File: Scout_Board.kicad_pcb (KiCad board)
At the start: 2 copper layers, 87.4 x 67 mm, 3 parts, among them J10 BBAI_P8, J2 Conn_02x07_Odd_Even, J9 BBAI_P9

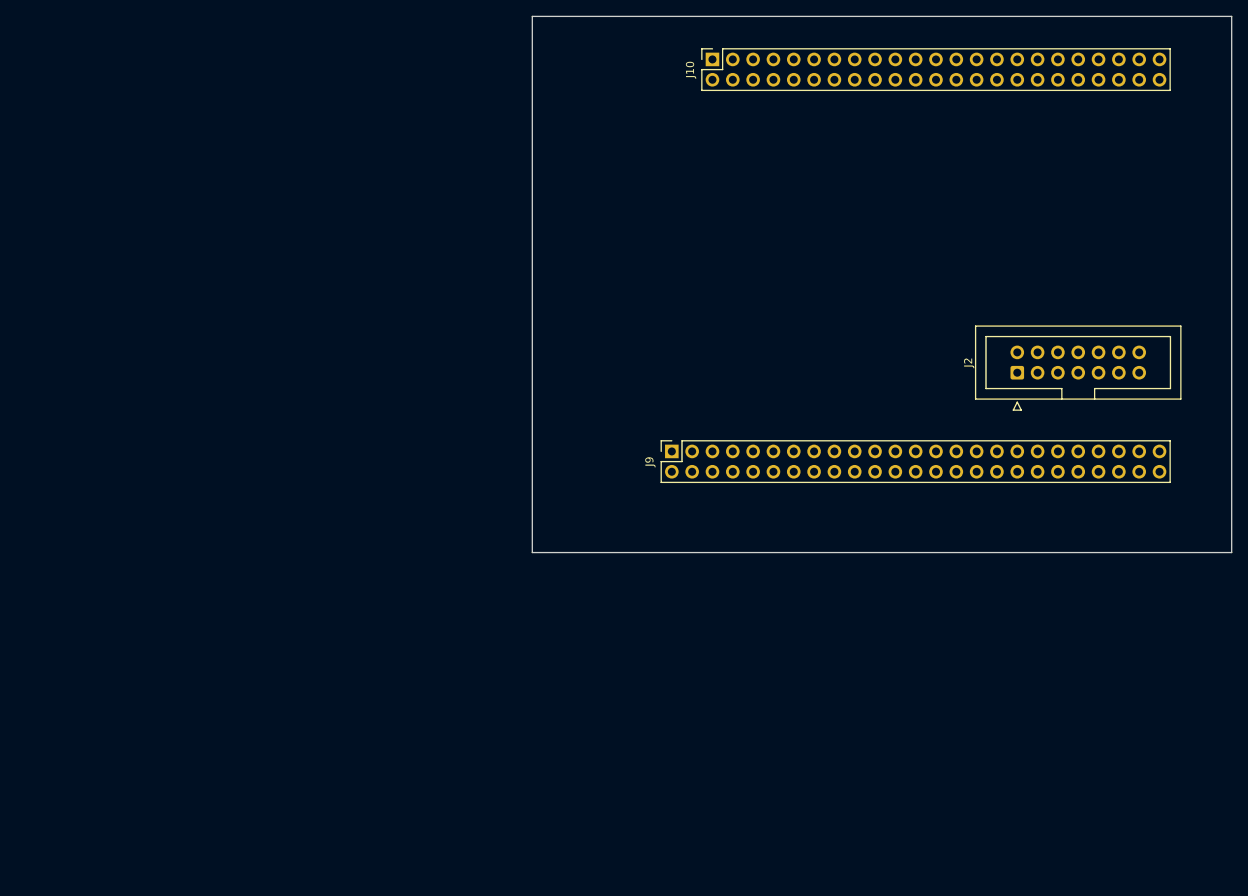
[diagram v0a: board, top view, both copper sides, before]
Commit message: New board test
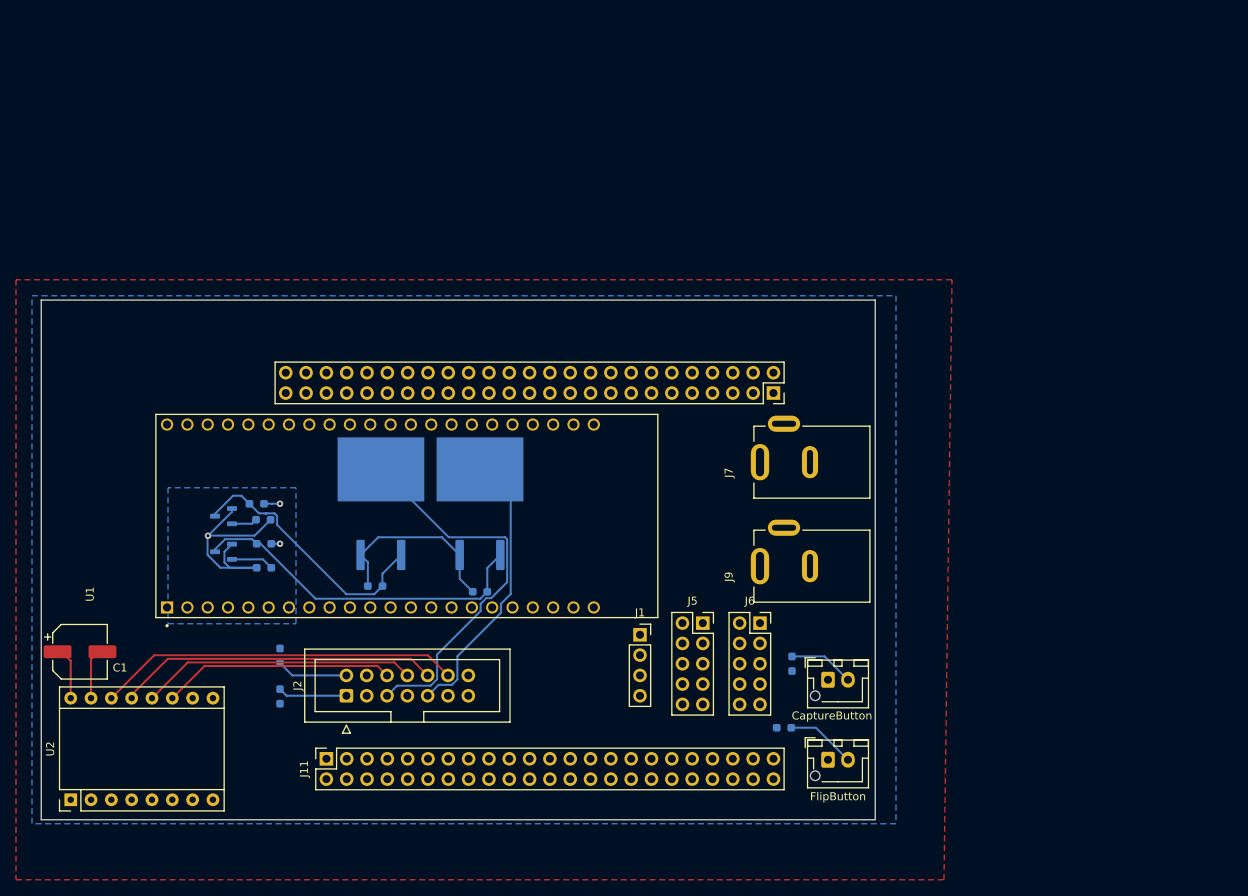
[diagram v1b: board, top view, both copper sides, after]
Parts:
- added C1: 100uF/16V, Capacitor_SMD:CP_Elec_6.3x5.9, F.Cu at (147.0, 169.5)
- added Conn2: CaptureButton, Connector_JST:JST_XH_B2B-XH-AM_1x02_P2.50mm_Vertical, F.Cu at (240.5, 173.0)
- added Conn4: FlipButton, Connector_JST:JST_XH_B2B-XH-AM_1x02_P2.50mm_Vertical, F.Cu at (240.5, 183.0)
- added J1: Conn_01x04_Pin, Connector_PinSocket_2.54mm:PinSocket_1x04_P2.54mm_Vertical, F.Cu at (217.0, 167.4)
- added J11: BBAI_P8, Connector_PinSocket_2.54mm:PinSocket_2x23_P2.54mm_Vertical, F.Cu at (177.8, 182.9)
- added J5: 5V, Connector_PinSocket_2.54mm:PinSocket_2x05_P2.54mm_Vertical, F.Cu at (224.8, 165.9)
- added J6: GND, Connector_PinSocket_2.54mm:PinSocket_2x05_P2.54mm_Vertical, F.Cu at (232.0, 165.9)
- added J7: IN, RAPC722X:SWITCHCRAFT_RAPC722X, F.Cu at (238.2, 145.8)
- added MOSFET1: IRFZ44NSTRLPBF, IRFZ44NSTRLPBF:DPAK254P1524X483-3N, B.Cu at (184.6, 151.0)
- added MOSFET2: IRFZ44NSTRLPBF, IRFZ44NSTRLPBF:DPAK254P1524X483-3N, B.Cu at (197.0, 151.0)
- added Q1: BSS138, BSS138:SOT95P240X111-3N, B.Cu at (164.9, 152.6)
- added Q2: BSS138, BSS138:SOT95P240X111-3N, B.Cu at (164.9, 157.0)
- added R1: 10k, Resistor_SMD:R_0603_1608Metric_Pad0.98x0.95mm_HandSolder, B.Cu at (235.0, 179.0)
- added R10: 1M, Resistor_SMD:R_0603_1608Metric_Pad0.98x0.95mm_HandSolder, B.Cu at (183.9, 161.3)
- added R11: 10k, Resistor_SMD:R_0603_1608Metric_Pad0.98x0.95mm_HandSolder, B.Cu at (169.1, 151.0)
- added R12: 10k, Resistor_SMD:R_0603_1608Metric_Pad0.98x0.95mm_HandSolder, B.Cu at (170.0, 159.0)
- added R13: 1M, Resistor_SMD:R_0603_1608Metric_Pad0.98x0.95mm_HandSolder, B.Cu at (197.0, 162.0)
- added R14: 10k, Resistor_SMD:R_0603_1608Metric_Pad0.98x0.95mm_HandSolder, B.Cu at (170.0, 156.0)
- added R2: 10k, Resistor_SMD:R_0603_1608Metric_Pad0.98x0.95mm_HandSolder, B.Cu at (236.0, 171.0)
- added R7: 10k, Resistor_SMD:R_0603_1608Metric_Pad0.98x0.95mm_HandSolder, B.Cu at (172.0, 175.1)
- added R8: 10k, Resistor_SMD:R_0603_1608Metric_Pad0.98x0.95mm_HandSolder, B.Cu at (172.0, 170.0)
- added R9: 10k, Resistor_SMD:R_0603_1608Metric_Pad0.98x0.95mm_HandSolder, B.Cu at (169.9, 153.0)
- added U1: ESP32-S3-DEVKITC-1U-N8R2, ESP32-S3-DEVKITC-1-N8R2:XCVR_ESP32-S3-DEVKITC-1-N8R2, F.Cu at (187.9, 152.5)
- added U2: ~, Module:Pololu_Breakout-16_15.2x20.3mm, F.Cu at (145.8, 188.0)
- J10: value BBAI_P8 -> BBAI_P9; footprint Connector_PinSocket_2.54mm:PinSocket_2x23_P2.54mm_Vertical -> Connector_PinSocket_2.54mm:PinSocket_2x25_P2.54mm_Vertical
- J9: value BBAI_P9 -> IN; footprint Connector_PinSocket_2.54mm:PinSocket_2x25_P2.54mm_Vertical -> RAPC722X:SWITCHCRAFT_RAPC722X
- moved J2 93.1 mm to (180.3, 175.0)
- moved J10 42.4 mm to (233.7, 137.2), turned to -90 degrees
- moved J9 22.4 mm to (238.2, 158.8)
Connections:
- net BLb renamed +12V
- J2 pad 3: Sw1b -> 5V
- J2 pad 4: Sw1b -> 5V
- J9 pad 1: unconnected-(J9-GND-Pad1) -> 5V
- J9 pad 2: unconnected-(J9-GND-Pad2) -> GND
- J9 pad 3: unconnected-(J9-3.3V-Pad3) -> GND
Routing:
- net TLa: track 0.00 -> 48.0 mm
- net 2B: track 0.00 -> 45.3 mm
- net BottomLightsHV: track 0.00 -> 43.6 mm
- net 2A: track 0.00 -> 40.1 mm
- net BLa: track 0.00 -> 35.2 mm
- net 1A: track 0.00 -> 34.4 mm
- net TopLightsHV: track 0.00 -> 33.2 mm
- net GND: track 0.00 -> 30.7 mm
- net +3.3V: track 0.00 -> 29.5 mm, vias 0 -> 1
- net 1B: track 0.00 -> 29.0 mm
- net Sw2: track 0.00 -> 8.94 mm
- net FlipButton: track 0.00 -> 8.74 mm
- net Sw1: track 0.00 -> 8.64 mm
- net CaptureButton: track 0.00 -> 8.21 mm
- net +12V: track 0.00 -> 6.98 mm
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- added copper zone on F.Cu, net +12V
- added copper zone on B.Cu, net +3.3V
- added copper zone on In1.Cu, net +3.3V
- added copper zone on In2.Cu, net 5V
- added copper zone on B.Cu, net GND
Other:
- board size 87.4 x 67 mm -> 104.2 x 65 mm
- copper layers 2 -> 4

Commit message: Layout changes
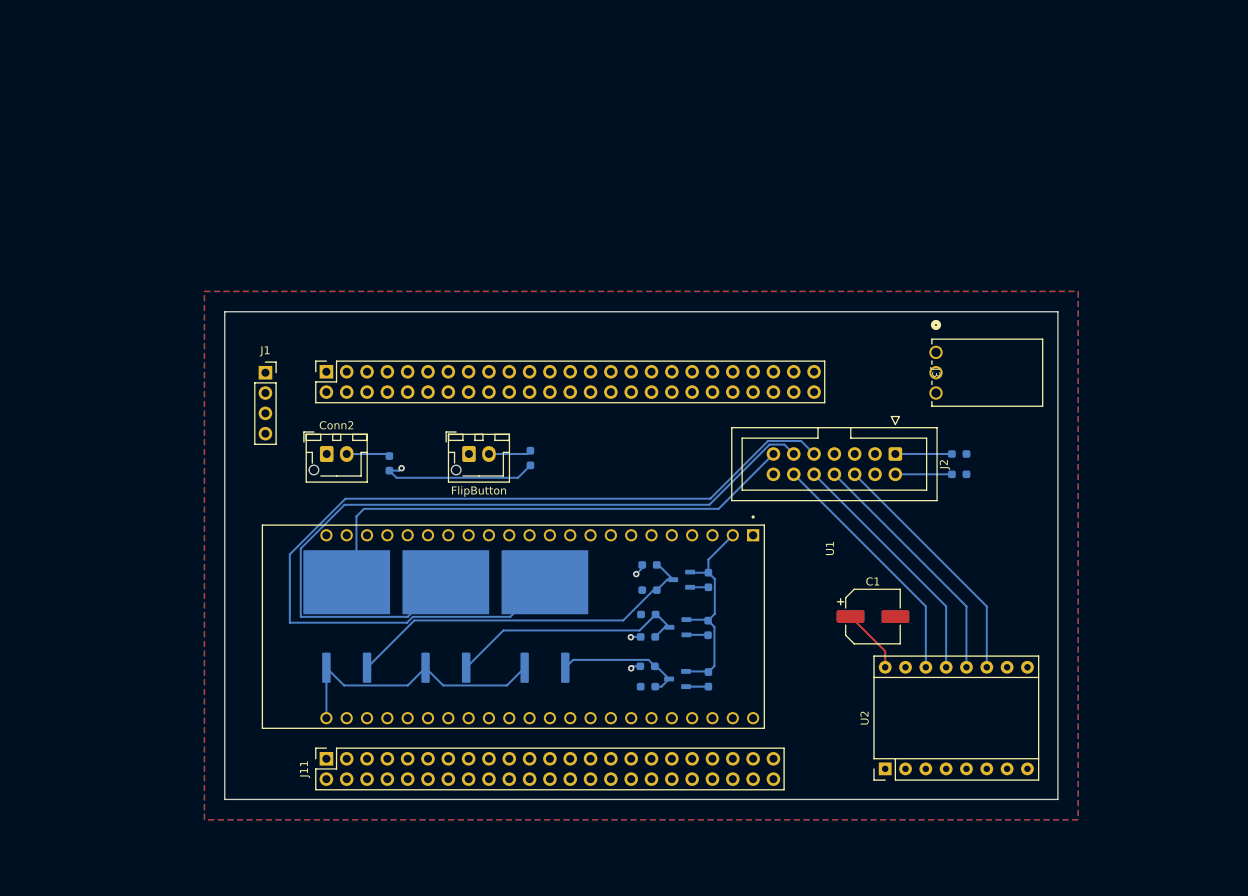
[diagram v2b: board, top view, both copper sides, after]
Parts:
- removed J5: 5V, Connector_PinSocket_2.54mm:PinSocket_2x05_P2.54mm_Vertical
- removed J6: GND, Connector_PinSocket_2.54mm:PinSocket_2x05_P2.54mm_Vertical
- removed J7, J9: IN, RAPC722X:SWITCHCRAFT_RAPC722X
- added J3: 705530002, 705530002:CONN3_53-0002_MOL, F.Cu at (254.0, 132.1)
- added MOSFET3: IRFZ44NSTRLPBF, IRFZ44NSTRLPBF:DPAK254P1524X483-3N, B.Cu at (180.3, 165.1)
- added Q3: BSS138, BSS138:SOT95P240X111-3N, B.Cu at (222.2, 160.5)
- added R29: 10k, Resistor_SMD:R_0603_1608Metric_Pad0.98x0.95mm_HandSolder, B.Cu at (225.6, 160.5)
- added R30: 1M, Resistor_SMD:R_0603_1608Metric_Pad0.98x0.95mm_HandSolder, B.Cu at (218.2, 158.6)
- added R31: 10k, Resistor_SMD:R_0603_1608Metric_Pad0.98x0.95mm_HandSolder, B.Cu at (218.2, 161.8)
- moved U2 101.9 mm to (247.7, 184.1)
- moved C1 99.2 mm to (246.1, 165.1)
- moved R7 90.1 mm to (256.9, 144.8), turned to 0 degrees
- moved R8 87.9 mm to (256.9, 147.3), turned to 0 degrees
- moved J2 75.0 mm to (248.9, 144.8), turned to -90 degrees
- moved Conn2 68.7 mm to (177.8, 144.8)
- moved Q1 60.3 mm to (221.7, 172.9)
- moved R9 59.1 mm to (225.6, 172.9), turned to -90 degrees
- moved Conn4 58.9 mm to (195.6, 144.8)
- moved Q2 57.6 mm to (221.7, 166.4)
- moved J1 57.1 mm to (170.2, 134.6)
- moved R2 56.2 mm to (185.7, 145.9)
- moved R12 56.0 mm to (225.5, 166.5), turned to -90 degrees
- moved J10 55.9 mm to (177.8, 134.5), turned to 90 degrees
- moved R11 54.0 mm to (218.0, 173.9), turned to 0 degrees
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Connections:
- J2 pad 11: +12V -> BL-
- J2 pad 13: unconnected-(J2-Pin_13-Pad13) -> UV-
- J2 pad 5: TLa -> +12V
- J2 pad 9: BLa -> TL-
- MOSFET1 pad 2: TLa -> TL-
- MOSFET2 pad 2: BLa -> BL-
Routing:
- net TL-: track 0.00 -> 114.6 mm
- net BL-: track 0.00 -> 96.0 mm
- net UV-: track 0.00 -> 64.1 mm
- net TLa: track 48.0 -> 0.00 mm
- net UVLightsHV: track 0.00 -> 45.6 mm
- net BLa: track 35.2 -> 0.00 mm
- net GND: track 30.7 -> 59.2 mm, vias 0 -> 4
- net TopLightsHV: track 33.2 -> 16.5 mm
- net 2B: track 45.3 -> 31.0 mm
- net BottomLightsHV: track 43.6 -> 31.1 mm
- net 2A: track 40.1 -> 31.0 mm
- net 1A: track 34.4 -> 31.0 mm
- net FlipButton: track 8.74 -> 5.35 mm
- net 5V: track 3.09 -> 0.00 mm, vias 2 -> 0
- net CaptureButton: track 8.21 -> 5.44 mm
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- added copper zone on In1.Cu, net +12V
- added copper zone on In2.Cu, net +3.3V
- added copper zone on B.Cu, net 5V
- added copper zone on F.Cu, net GND
- removed copper zone on F.Cu, net +12V
- removed copper zone on B.Cu, net +3.3V
- removed copper zone on In1.Cu, net +3.3V
- removed copper zone on In2.Cu, net 5V
- removed copper zone on B.Cu, net GND
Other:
- board size 104.2 x 65 mm -> 104.1 x 61 mm
